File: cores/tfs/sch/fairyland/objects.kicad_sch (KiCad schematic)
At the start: 88 parts, among them IC1 74LS04, IC10 27128, IC11 27128, IC12 74LS194, IC13 74LS194, IC14 74LS74, IC15 74LS08, IC16 74LS86, IC18 74LS161, IC2 74LS107, IC20 74LS139, IC21 74LS298, IC22 74LS194, IC23 74LS194, IC24 74LS74, IC25 74LS10, IC26 74LS86, IC27 74LS161, IC28 74LS161, IC30 74LS86, IC31 74LS298, IC32 27128, IC33 27128, IC34 27128, IC35 27128, IC36 74LS158, IC37 74LS04, IC38 74LS86, IC39 74LS86, IC40 74LS20, IC41 74LS373, IC42 74LS373, IC43 74LS273, IC45 74LS245, IC46 74LS273, IC47 74LS04, IC47 74LS273, IC48 74LS374, IC49 74LS244, IC5 74LS74, IC50 74LS669, IC51 74LS669, IC52 74LS273, IC53 74LS32, IC54 74LS273, IC55 74LS273, IC56 74LS283, IC57 74LS283, IC58 MBM2148, IC59 MBM2148, IC6 74LS86, IC60 74LS244, IC61 74LS298, IC62 74LS298, IC63 74LS374, IC67 MBM2148, IC68 74LS08, IC69 74LS257, IC7 74LS298, IC70 74LS42, IC75 74LS244, IC76 MBM2148, IC77 MBM2148, IC78 MBM2148, IC8 27128, IC82 74LS244, IC83 74LS157, IC84 74LS157, IC85 74LS157, IC86 RAM_2016, IC9 27128, IC90 74LS245, IC91 74LS245, IC92 74LS174, IC93 74LS174, IC94 74LS245, IC95 74LS374, IC96 74LS08

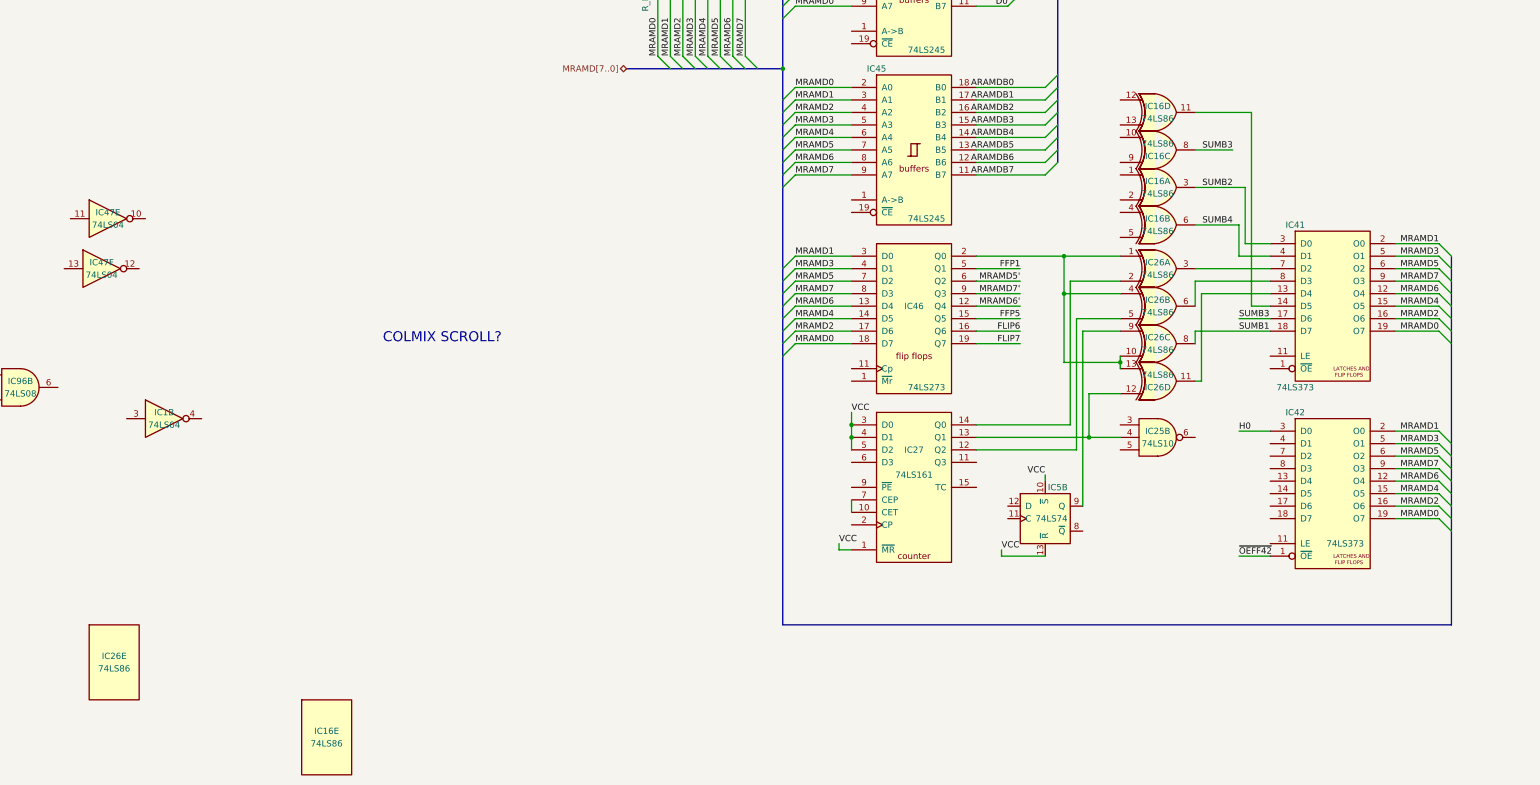
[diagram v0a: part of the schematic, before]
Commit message: wip fairyland video
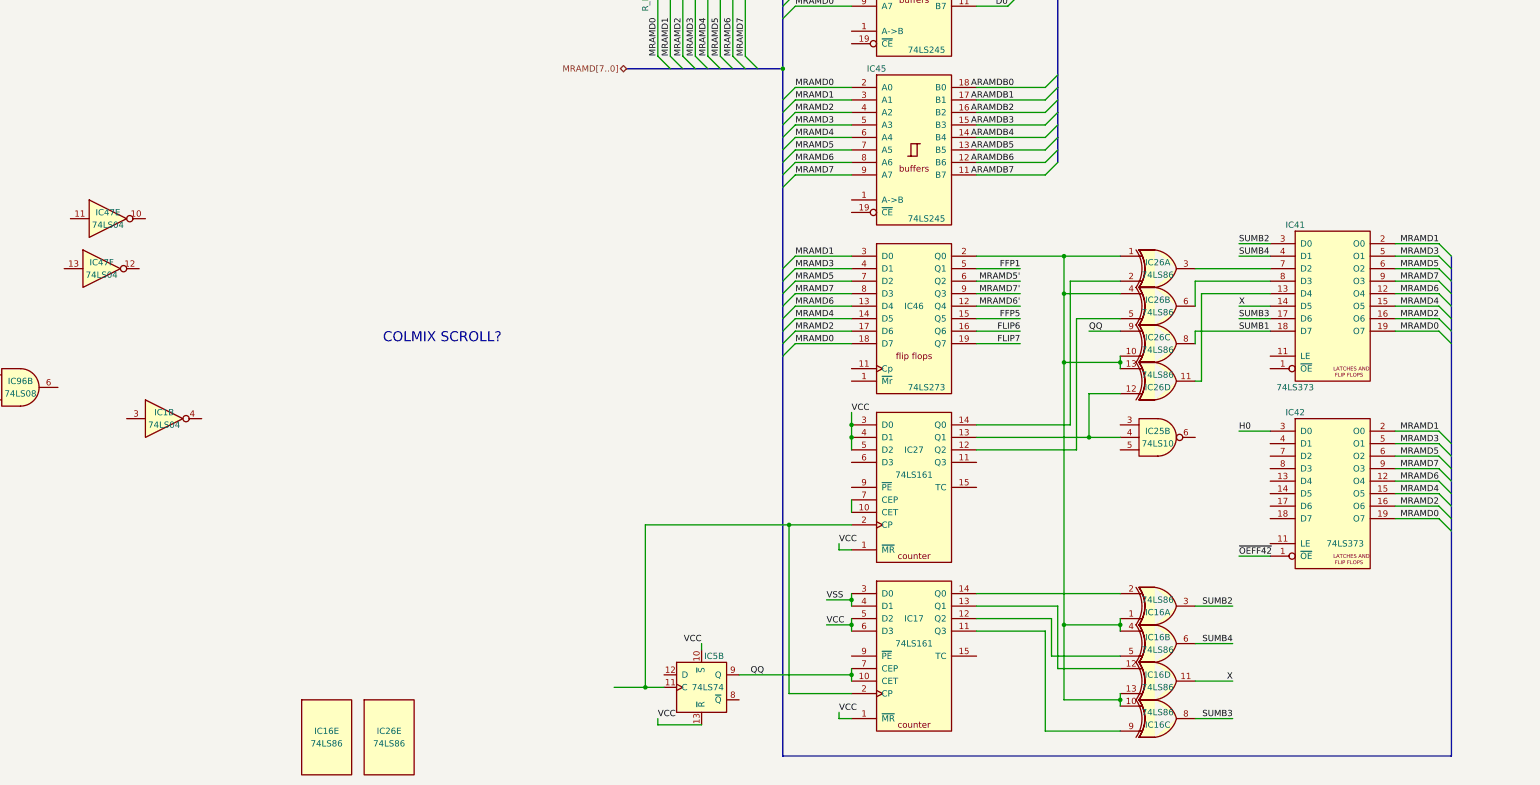
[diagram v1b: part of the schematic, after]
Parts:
- added IC17: 74LS161, symbol jt74:74LS161
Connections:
- net VCC: now also IC17.1 (~{MR}), IC17.5 (D2), IC17.6 (D3)
- net VSS: now also IC17.3 (D0), IC17.4 (D1)
- net at IC5.11 (C): now also IC27.2 (CP), IC17.2 (CP)
- net QQ: now reaches IC26.9, IC5.9 (Q)
- net QQ: now also IC17.10 (CET), IC17.7 (CEP)
- net at IC16.10: now also IC16.1, IC16.13, IC16.4, IC26.1, IC26.10, IC26.13, IC26.4, IC46.2 (Q0)
- net at IC16.9: now also IC17.11 (Q3)
- net at IC16.2: now also IC17.14 (Q0)
- net X: now reaches IC16.11, IC41.14 (D5)
- net at IC16.12: now also IC17.13 (Q1)
- net at IC16.5: now also IC17.12 (Q2)
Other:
- moved on the sheet: IC16A, IC16B, IC16C, IC16D, IC26E, IC5B
